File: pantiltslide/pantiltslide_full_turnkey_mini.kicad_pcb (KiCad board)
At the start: 4 copper layers, 54 x 93 mm, 63 parts, among them J1 Conn_01x22_Socket, J17 Motor_Slide, J18 Motor_Pan, J19 Motor_Tilt, J2 Conn_01x22_Socket, J20 TCA9548A_Mux, J21 AS5600_Pan, J22 AS5600_Tilt, J23 OLED, J24 TCA9548A_Mux, J26 Limit_Min, J27 Limit_Max, J28 Motor_Aux, J29 Enc_Slide, J3 MUX_2, J30 Enc_Pan, J31 Enc_Tilt, J32 Enc_Aux, J33 Btn_SetKeyframe, J34 Btn_ClearKeyframe, J35 Btn_PlayPause, J36 Btn_Reset, J37 5V_In, J38 24V_In, J4 MUX_3, J41 Aux_Max, J5 MUX_4, J6 MUX_5, J7 MUX_6, J8 MUX_7, U1 tmc2209, U2 tmc2209, U3 tmc2209, U4 tmc2209

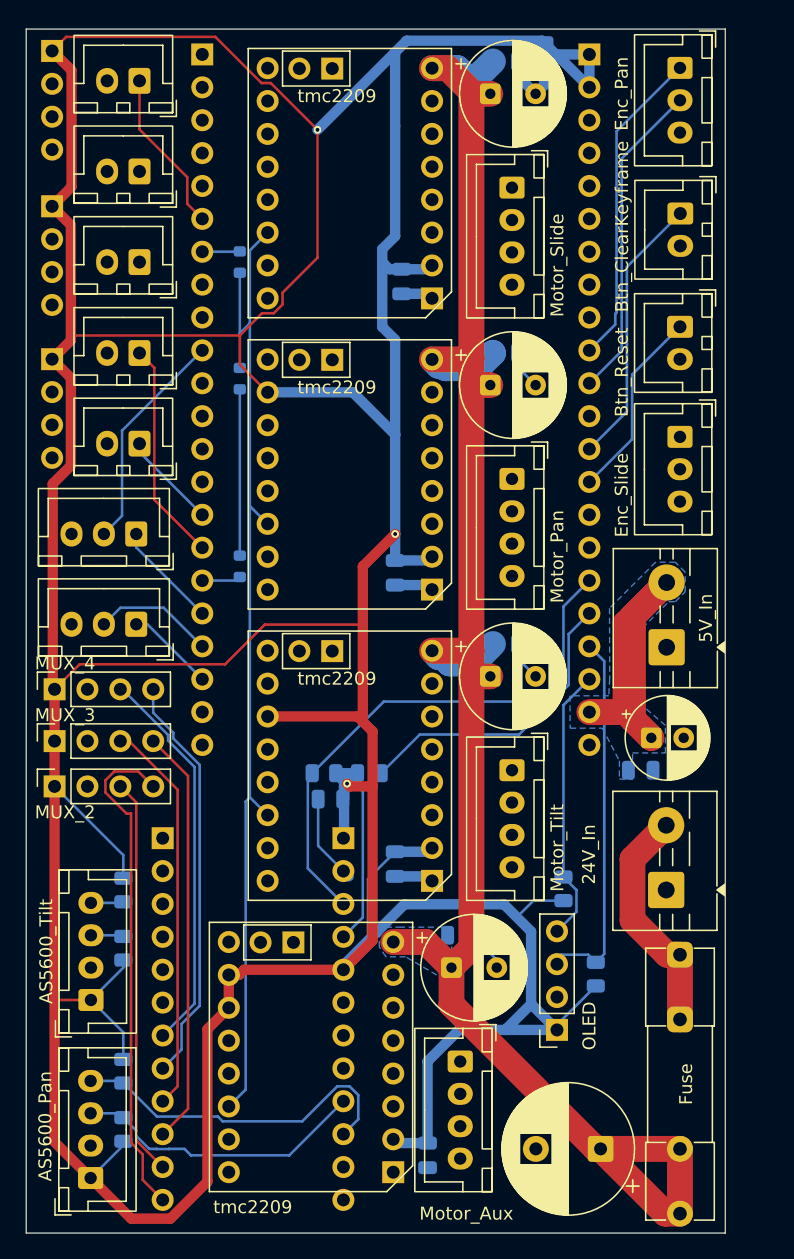
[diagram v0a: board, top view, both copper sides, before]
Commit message: re wiring pcb
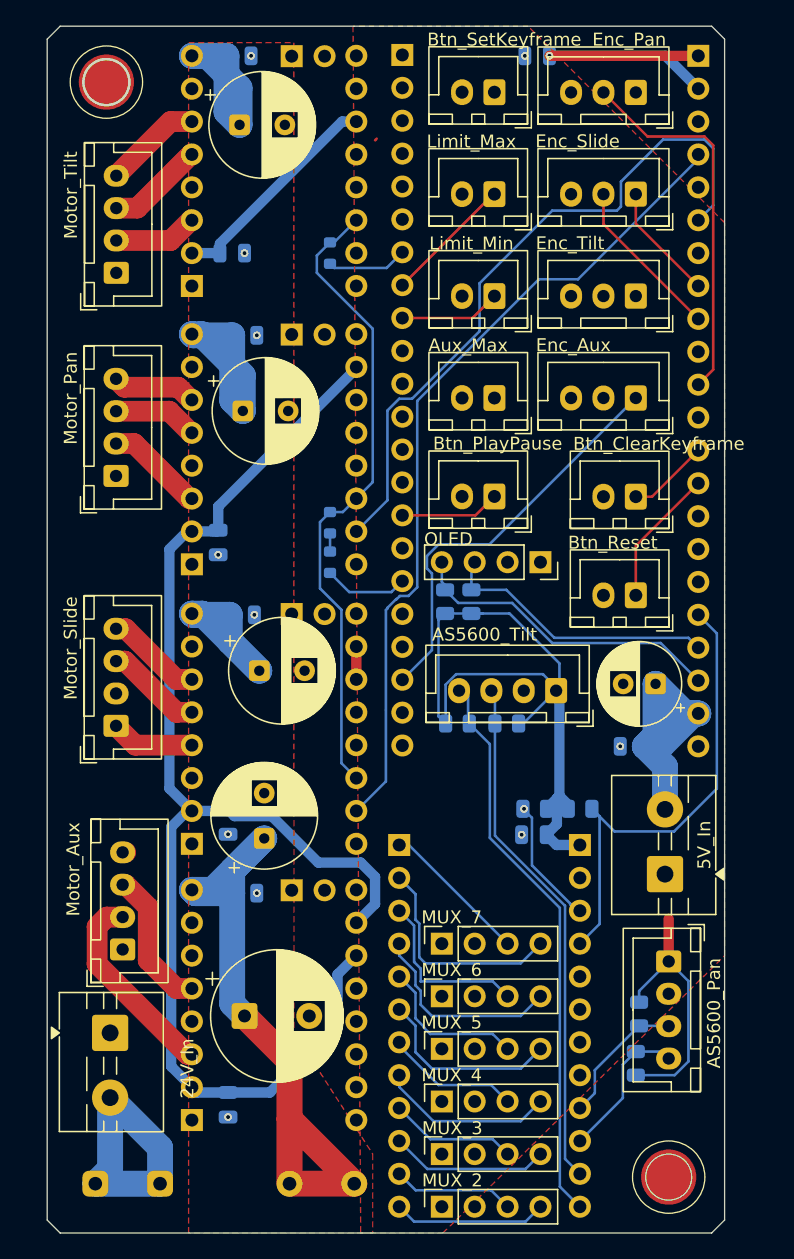
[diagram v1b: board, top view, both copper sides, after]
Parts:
- F1, U1, U2, U3, U4: moved to B.Cu
- J6, J7, J8: moved to F.Cu
- moved J8 75.2 mm to (117.6, 88.6), turned to 90 degrees
- moved J7 68.0 mm to (117.6, 92.7), turned to 90 degrees
- moved C13 65.0 mm to (101.1, 101.1)
- moved J6 61.2 mm to (117.6, 96.8), turned to 90 degrees
- moved J17 51.6 mm to (92.4, 71.8), turned to 90 degrees
- moved C8 49.9 mm to (101.9, 20.1)
- moved U3 49.6 mm to (98.3, 37.8), turned to 0 degrees
- moved J19 49.1 mm to (92.5, 36.8), turned to 90 degrees
- moved C15 48.8 mm to (101.4, 35.3), turned to 0 degrees
- moved F1 48.5 mm to (90.8, 107.2), turned to 0 degrees
- moved C2 48.0 mm to (103.5, 67.6)
- moved J21 47.7 mm to (135.1, 90.0), turned to -90 degrees
- moved C6 47.3 mm to (102.2, 63.2)
- moved C4 46.8 mm to (102.0, 25.4)
- moved U1 46.0 mm to (98.3, 80.9), turned to 0 degrees
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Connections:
- J3 pad 2: unconnected-(J3-Pin_2-Pad2) -> GND
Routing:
- net 3.3v: track 462.4 -> 225.3 mm, vias 3 -> 2
- net MUX_CH7_SDA: track 62.7 -> 11.5 mm
- net MUX_CH7_SCL: track 61.0 -> 17.0 mm
- net GPIO_5: track 28.4 -> 72.4 mm
- net MUX_CH6_SDA: track 56.7 -> 13.3 mm
- net +24V: track 143.2 -> 100.6 mm
- net MUX_CH6_SCL: track 52.5 -> 15.6 mm
- net GPIO_4: track 29.0 -> 64.0 mm
- net MUX_CH5_SDA: track 45.6 -> 11.9 mm
- net MUX_CH5_SCL: track 46.4 -> 14.6 mm
- net GND: track 30.4 -> 2.54 mm, vias 0 -> 11
- net MUX_CH2_SCL: track 38.9 -> 11.9 mm
- net GPIO_1: track 83.3 -> 109.0 mm
- net GPIO_21: track 8.42 -> 34.0 mm
- net GPIO_19: track 6.86 -> 31.9 mm
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- added copper zone on F.Cu, net +24V
- added copper zone on F.Cu, net 3.3v
- removed copper zone on B.Cu, net +24V
- removed copper zone on B.Cu, net VCC_5V
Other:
- board size 54 x 93 mm -> 52.3 x 93.2 mm
